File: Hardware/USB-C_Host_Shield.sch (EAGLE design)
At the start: 23 parts, among them U1 ARDUINO_UNO_R3_SHIELDBASIC, U4 AP7361C-33FGEUDFN-8, U5 MAX3421

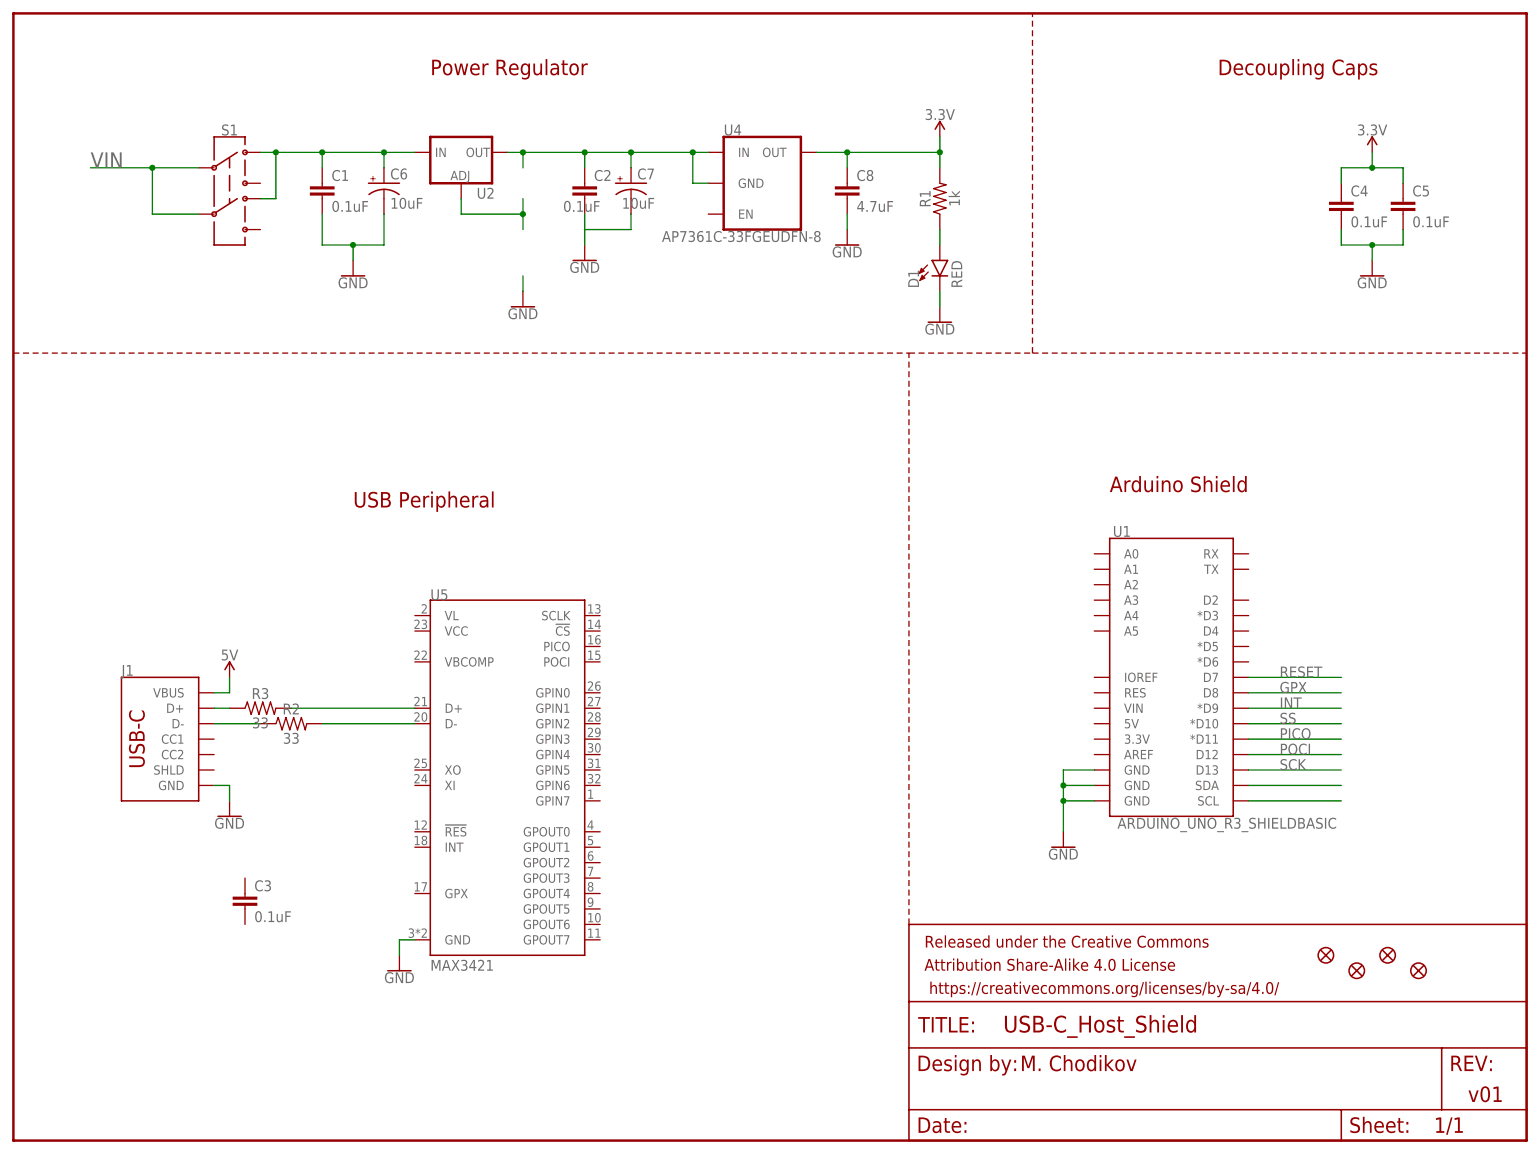
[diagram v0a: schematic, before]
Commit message: Updated schematic
Continued work on schematic - shelving project for a little to define requirements a little more clearly
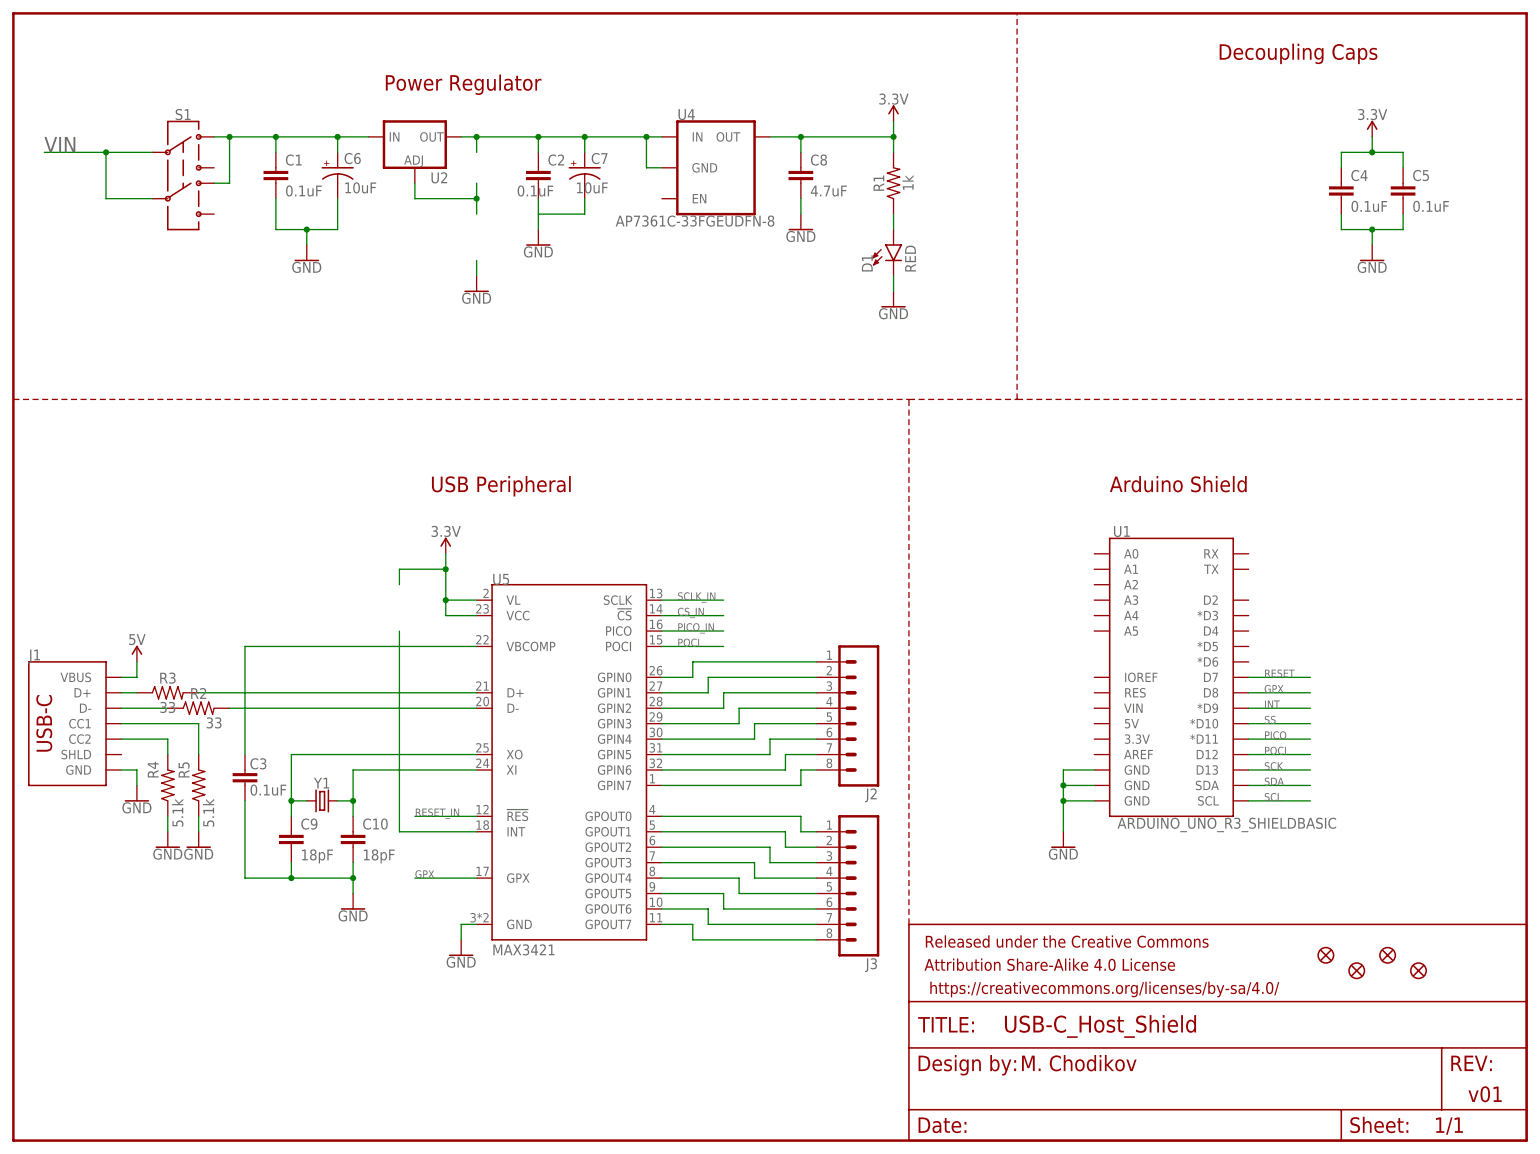
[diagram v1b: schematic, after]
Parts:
- added C10, C9: 18pF, SparkFun-Capacitors:18PF-0603-50V-5%
- added J2, J3: (no value), SparkFun-Connectors:CONN_08"
- added R4, R5: 5.1k, SparkFun-Resistors:5.1KOHM5.1KOHM-0603-1/10W-1%
- added Y1: (no value), SparkFun-Clocks:CRYSTAL-12MHZ
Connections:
- net N$15 renamed SDA
- net N$16 renamed SCL
- new net CS_IN: U5.!CS
- new net N$12: J3.1, U5.GPOUT0
- new net N$13: J3.2, U5.GPOUT1
- new net N$14: J3.3, U5.GPOUT2
- new net N$15: J1.CC1, R5.2
- new net N$16: J1.CC2, R4.2
- new net N$17: J3.4, U5.GPOUT3
- new net N$18: J3.5, U5.GPOUT4
- new net N$19: J3.6, U5.GPOUT5
- new net N$20: J3.7, U5.GPOUT6
- new net N$21: J3.8, U5.GPOUT7
- new net N$22: J2.8, U5.GPIN7
- new net N$23: J2.7, U5.GPIN6
- new net N$24: J2.6, U5.GPIN5
- new net N$25: J2.5, U5.GPIN4
- new net N$26: J2.4, U5.GPIN3
- new net N$27: J2.3, U5.GPIN2
- new net N$28: J2.2, U5.GPIN1
- new net N$29: J2.1, U5.GPIN0
- new net N$34: C9.1, U5.XO, Y1.1
- new net N$35: U5.INT
- new net N$36: C10.1, U5.XI, Y1.2
- new net N$37: C3.1, U5.VBCOMP
- new net PICO_IN: U5.PICO
- new net RESET_IN: U5.!RES
- new net SCLK_IN: U5.SCLK
- net 3.3V: now also U5.VCC, U5.VL
- net GND: now also C10.2, C3.2, C9.2, R4.1, R5.1
- net GPX: now also U5.GPX
- net POCI: now also U5.POCI
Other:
- moved on the sheet: C1, C2, C3, C4, C5, C6, C7, C8, D1, J1, R1, R2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

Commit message: Continued work on Layout
Verify again 9/21 morning, but this should be nearly ready for layout
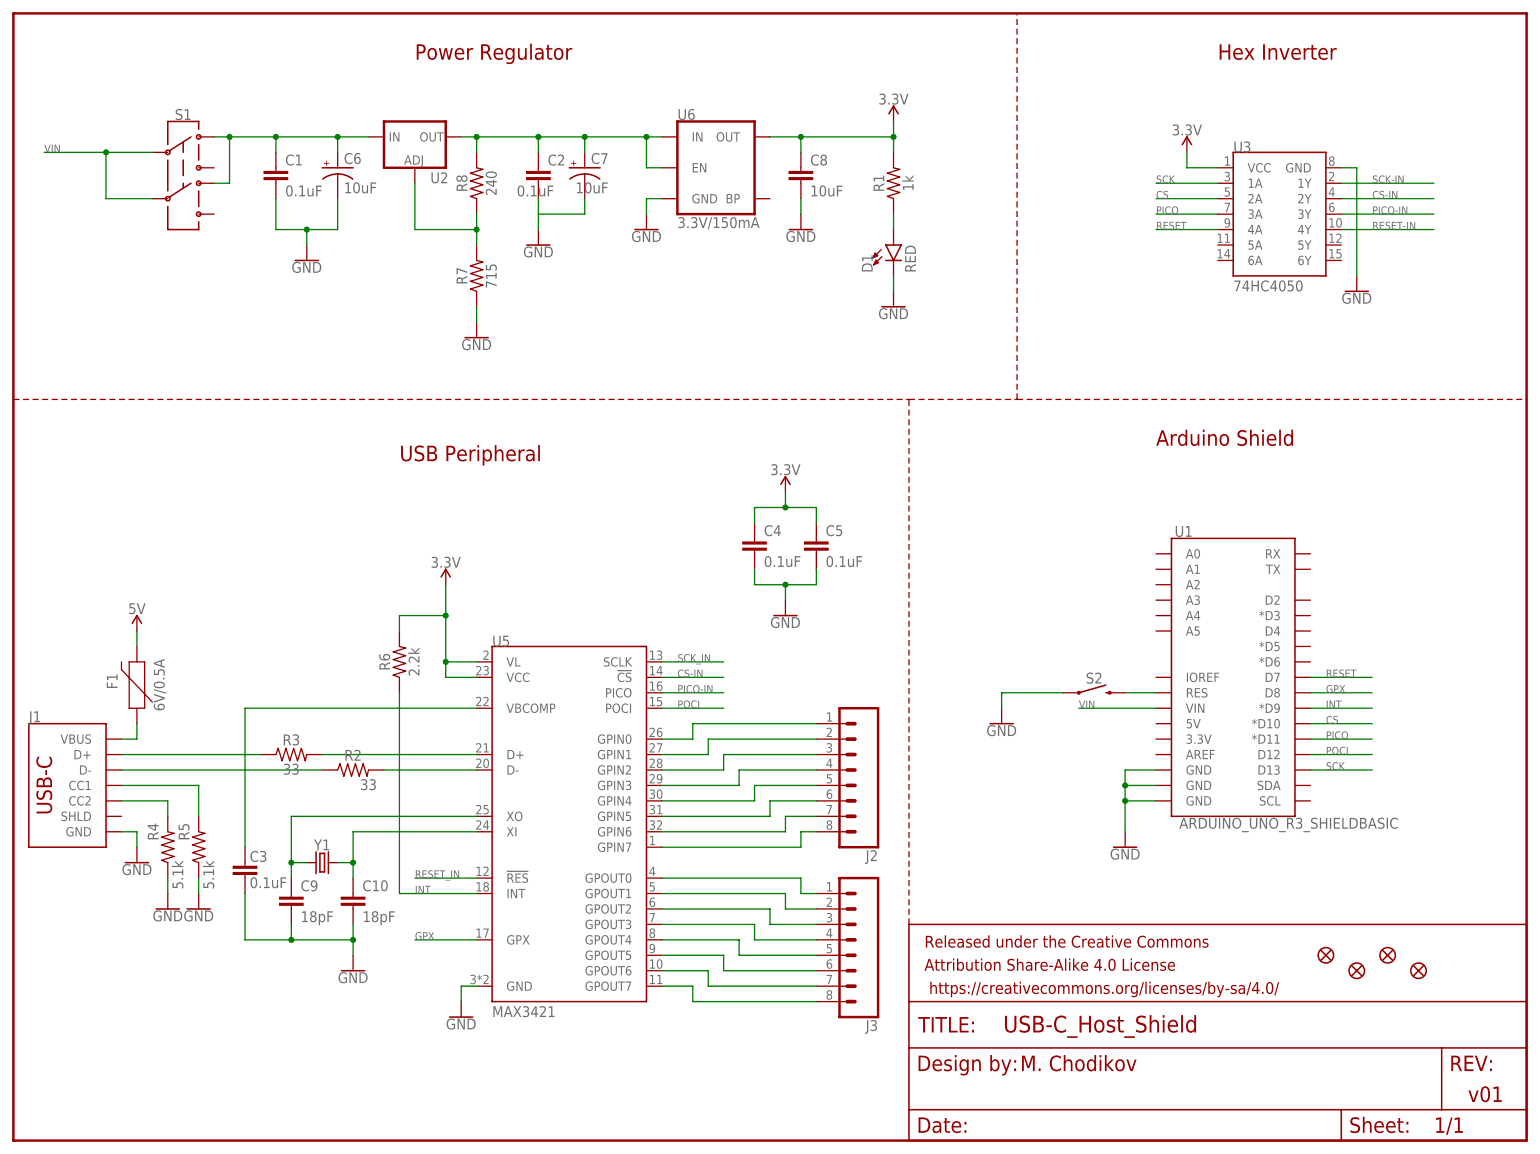
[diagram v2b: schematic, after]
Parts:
- removed U4: AP7361C-33FGEUDFN-8, SparkFun-IC-Power:AP7361C-33FGEUDFN-8
- added F1: 6V/0.5A, SparkFun-Fuses:PPTC_6V500MA-2
- added R6: 2.2k, SparkFun-Resistors:2.2KOHM-0603-1/10W-1%
- added R7: 715, SparkFun-Resistors:715OHM-0603-1/10W-1%
- added R8: 240, SparkFun-Resistors:240OHM-0603-1/10W-1%
- added S2: MOMENTARY-SWITCH-SPST-SMD-5.2MM-TALL, SparkFun-Switches:MOMENTARY-SWITCH-SPST-SMD-5.2MM-TALL
- added U3: 74HC4050, SparkFun-IC-Comms:HEX_CONVERTER
- added U6: 3.3V/150mA, SparkFun-IC-Power:V_REG_MIC52053.3V
- C8: value 4.7uF -> 10uF; device SparkFun-Capacitors:4.7UF-0603-6.3V-(10%) -> SparkFun-Capacitors:10UF-0603-6.3V-20%
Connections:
- net SCLK_IN renamed SCK_IN
- removed net CS_IN: U5.!CS
- removed net N$35: U5.INT
- removed net PICO_IN: U5.PICO
- removed net SCL: U1.SCL
- removed net SDA: U1.SDA
- removed net SS: U1.*D10
- new net CS: U1.*D10, U3.2A
- new net CS-IN: U3.2Y, U5.!CS
- new net N$30: S2.2, U1.RES
- new net N$31: F1.1, J1.VBUS
- new net N$5: R7.1
- new net PICO-IN: U3.3Y, U5.PICO
- new net RESET-IN: U3.4Y
- new net SCK-IN: U3.1Y
- net 3.3V: now also R6.2, U3.VCC, U6.OUT; no longer U4.OUT
- net 5V: now also F1.2; no longer J1.VBUS
- net GND: now also S2.1, U3.GND, U6.GND
- net INT: now also R6.1, U5.INT
- net N$3: now also R8.2, U6.EN, U6.IN; no longer U4.GND, U4.IN
- net N$4: now also R7.2, R8.1
- net PICO: now also U3.3A
- net RESET: now also U3.4A
- net SCK: now also U3.1A
- net VIN: now also U1.VIN
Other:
- note added: "Hex Inverter"
- note removed: "Decoupling Caps"
- moved on the sheet: C10, C3, C4, C5, C9, J1, J2, J3, R2, R3, R4, R5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
